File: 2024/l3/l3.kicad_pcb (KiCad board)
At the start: 2 copper layers, 137.5 x 129.1 mm, 23 parts, among them J1 Conn_01x04, SW1 SW_SPDT, SW2 SW_SPDT, SW3 SW_SPDT, SW4 SW_SPDT, U4 DEV-15583

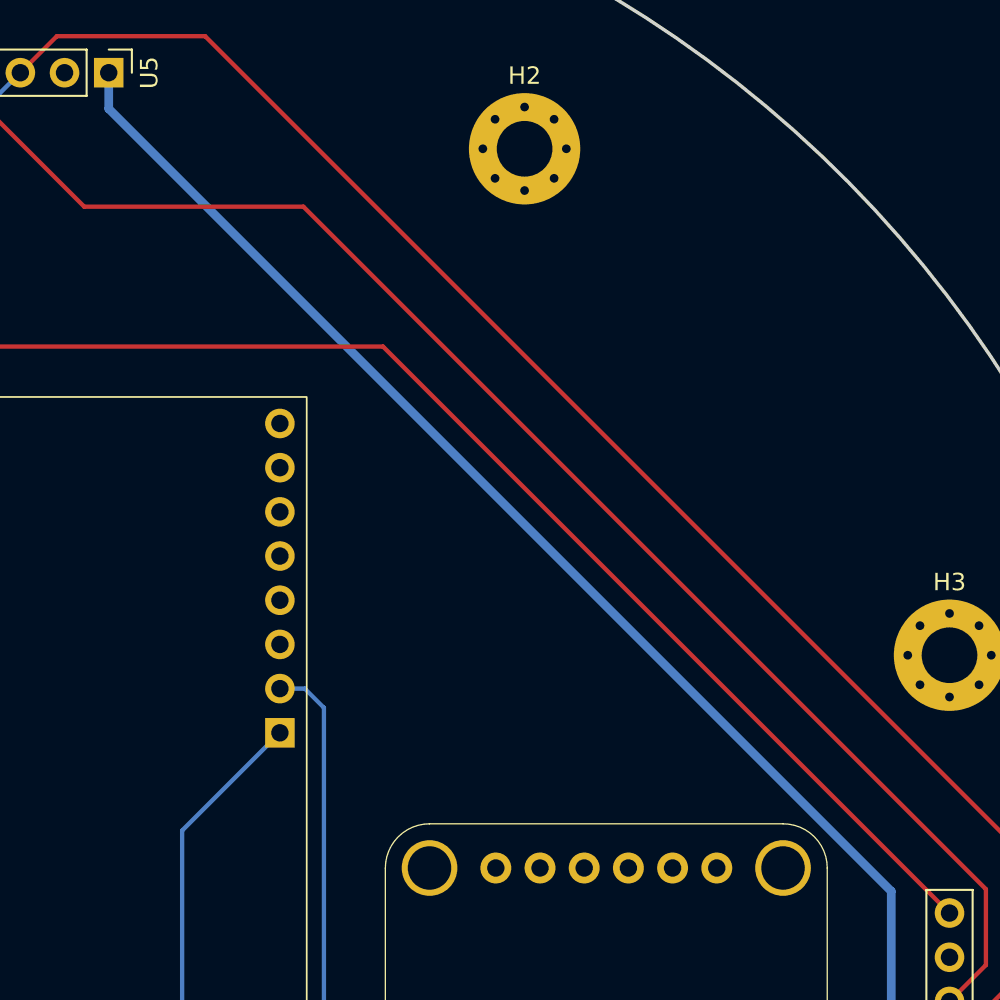
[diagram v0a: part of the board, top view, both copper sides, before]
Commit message: remove trace test
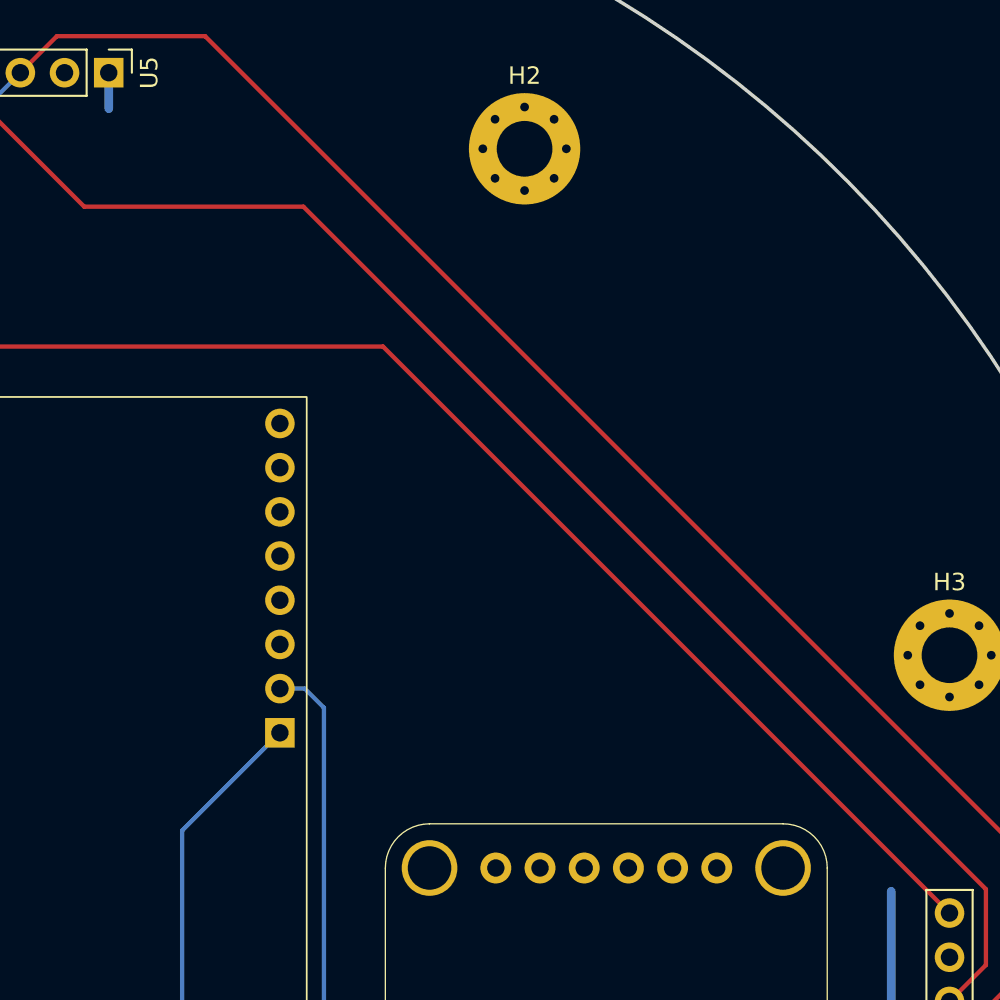
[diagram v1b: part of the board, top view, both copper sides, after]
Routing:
- net +5V: track 304.9 -> 241.3 mm
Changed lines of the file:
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@@
-	)
-	(segment
-		(start 111.4 44.07)
-		(end 156.38 89.05)
-		(width 0.5)
-		(layer "B.Cu")
-		(net 3)
 	)
 	(segment
